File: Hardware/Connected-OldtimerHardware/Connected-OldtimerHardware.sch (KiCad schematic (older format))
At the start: 25 parts, among them J1 NextionConnector, J2 MainConnector, J3 CAN_Bus_Connector, J4 AUXConnector, Q1 2N3906, U1 ParticleElectron, U2 TSR_2-2450, U3 CANTranceiverModule, U4 AdafruitFRAM, U5 AdafruitUltimateGPS, U6 MotionSensor, U7 SFH618A-2

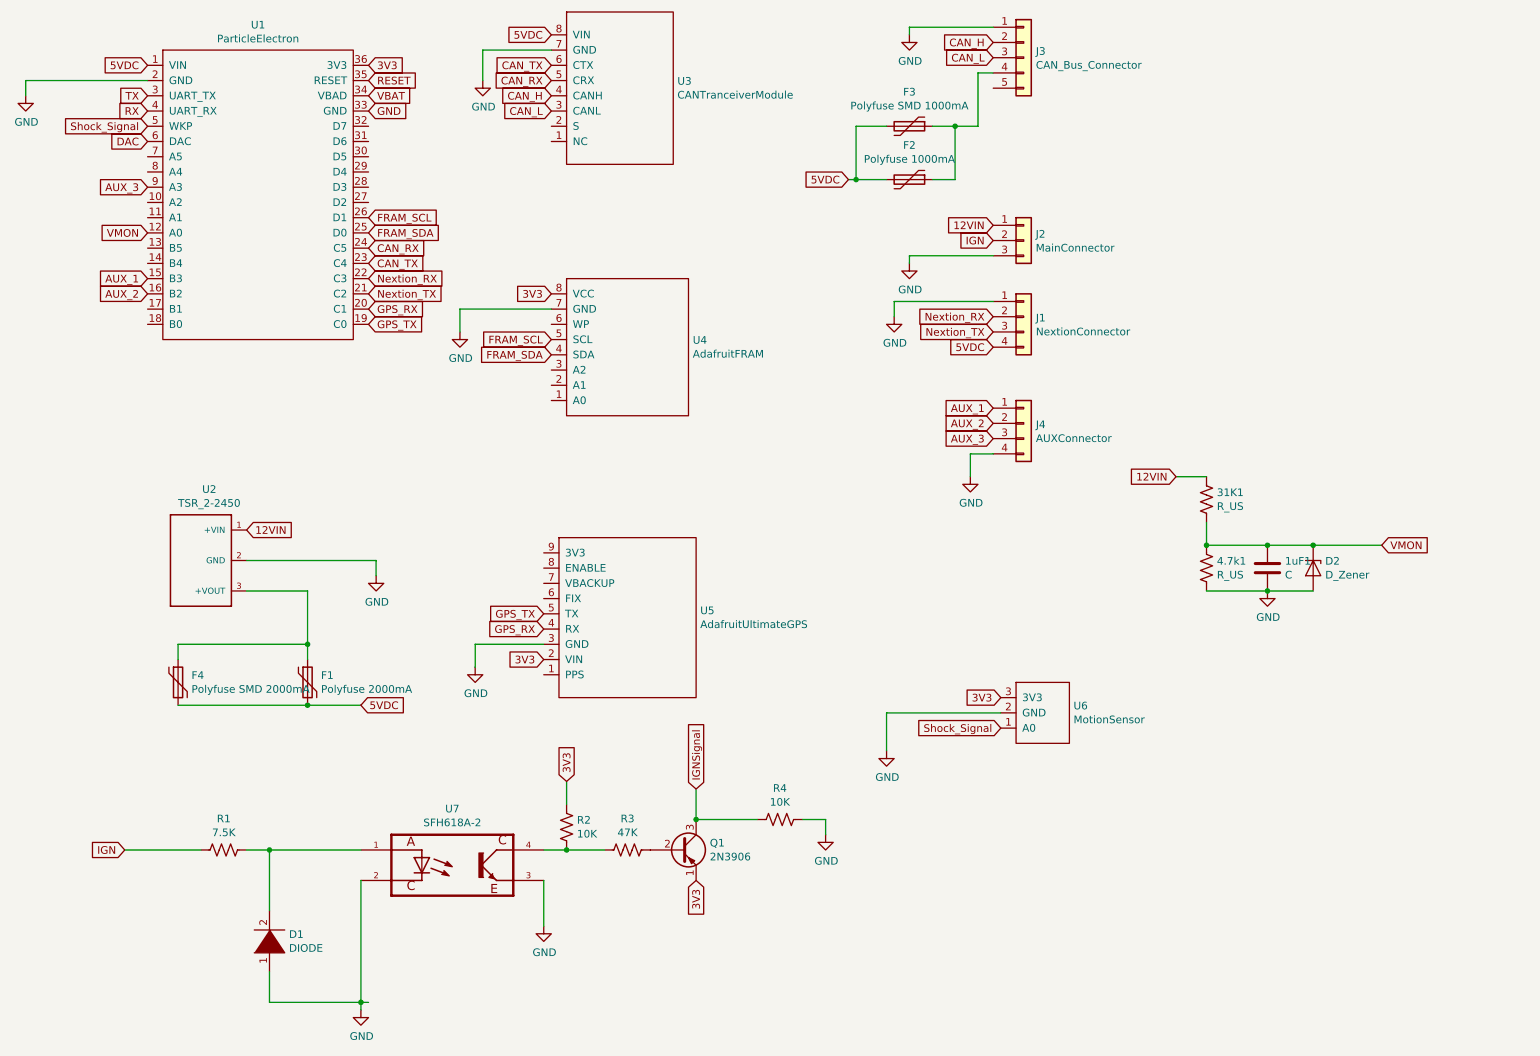
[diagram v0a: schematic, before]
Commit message: Generated Gerbers
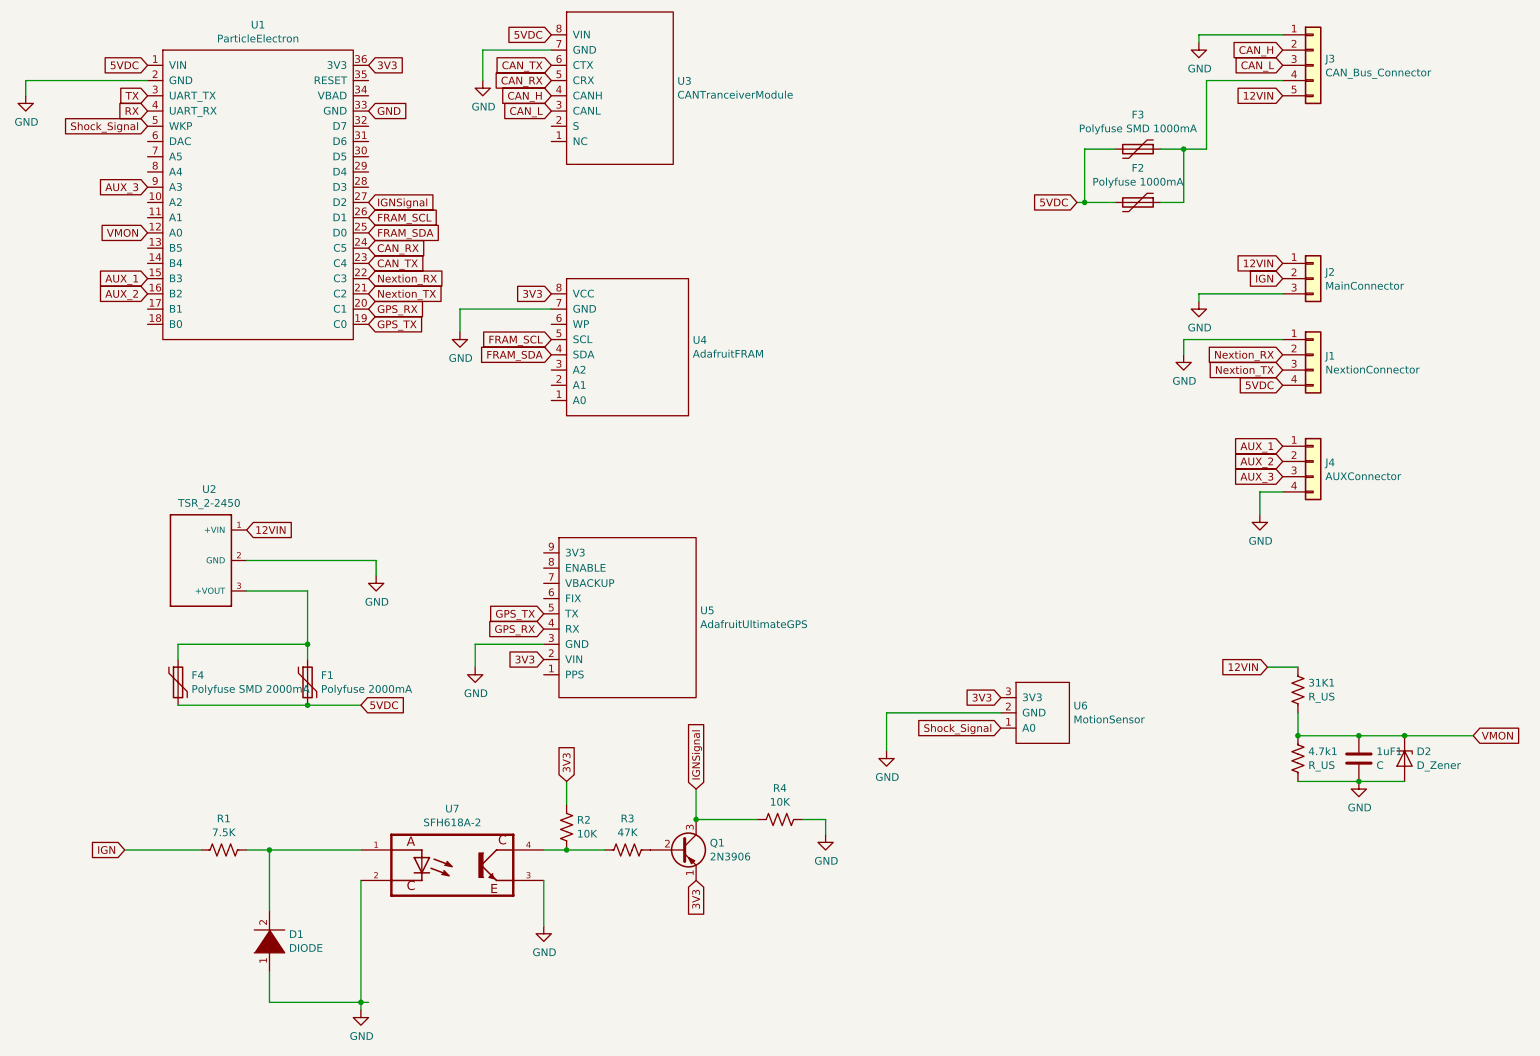
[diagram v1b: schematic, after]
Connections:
- net 12VIN: now also J3.5 (Pin_5)
- net IGNSignal: now also U1.27 (D2)
- net DAC: no longer names the net of U1.6 (DAC)
- net RESET: no longer names the net of U1.35 (RESET)
- net VBAT: no longer names the net of U1.34 (VBAD)
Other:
- moved on the sheet: 1uF1, 31K1, 4.7k1, D2, F2, F3, J1, J2, J3, J4
